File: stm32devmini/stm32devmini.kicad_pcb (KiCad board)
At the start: 2 copper layers, 52.1 x 20.3 mm, 30 parts, among them J1 USB_C_Receptacle_USB2.0, U1 XC6206P332MR, U2 STM32F103C8Tx, Y1 8M, Y2 32.768k

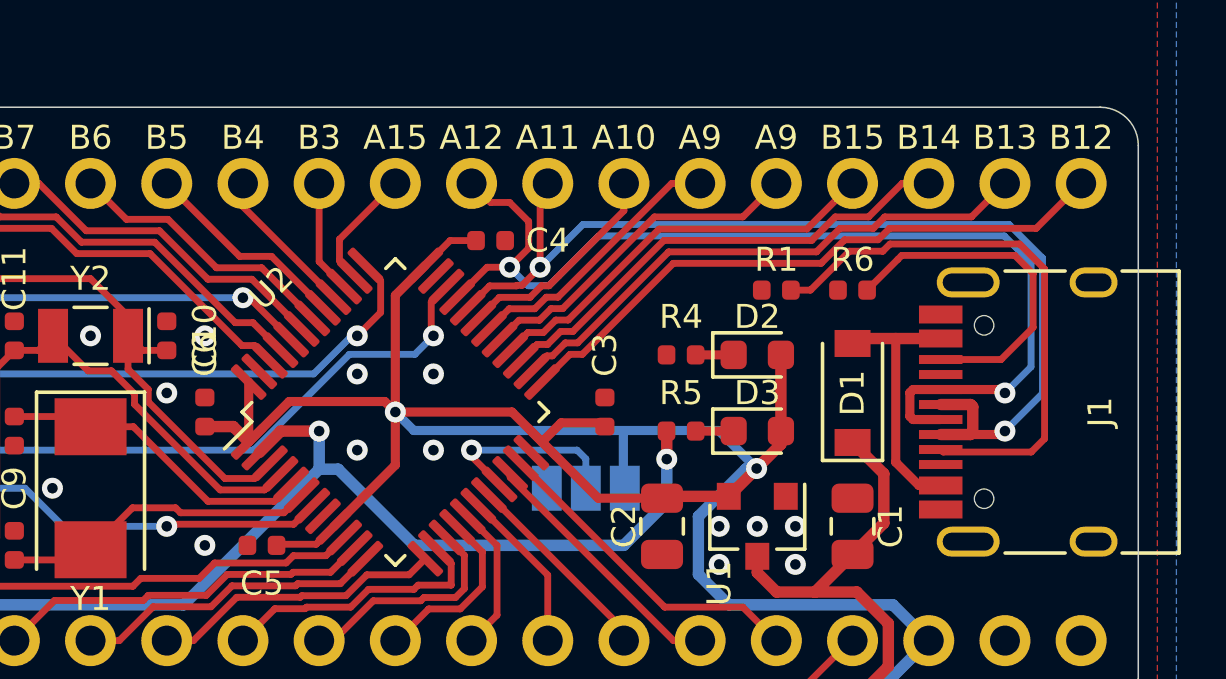
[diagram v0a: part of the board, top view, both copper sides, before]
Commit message: Hmmm
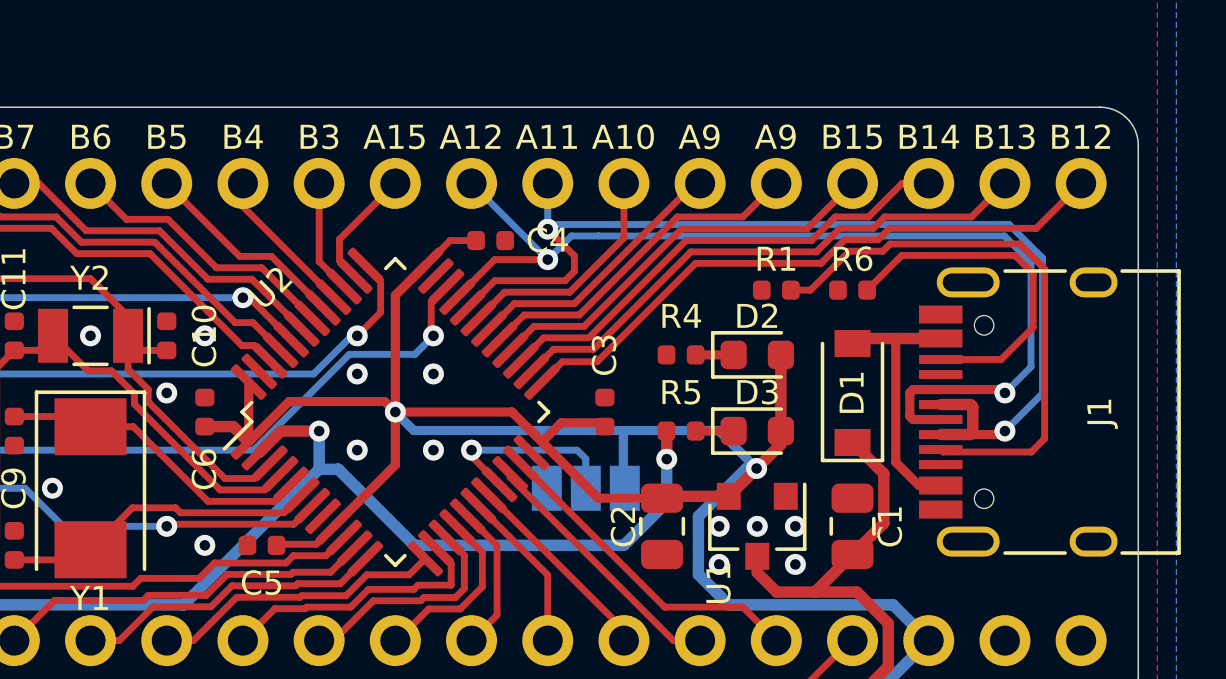
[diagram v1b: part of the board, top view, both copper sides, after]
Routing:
- net A11: track 35.2 -> 36.3 mm
- net A12: track 34.9 -> 34.0 mm
- net A10: track 7.25 -> 7.78 mm
